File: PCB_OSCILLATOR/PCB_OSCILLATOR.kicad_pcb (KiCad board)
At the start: 2 copper layers, 67 parts, among them J1 Jumper, J10 Jumper, J11 Jumper, J2 Jumper, J3 Jumper, J4 Jumper, J5 Jumper, J6 Jumper, J7 Jumper, J8 Jumper, J9 Jumper, P1 POWER SUPPLY, P2 SPI_AD5270_1, P3 SPI_AD5270_2, P4 SPI_AD9833_1, P5 SPI_AD9833_2, U1 AD5270, U2 AD8421, U3 AD9833, U4 AD5270, U5 AD8421, U6 AD9833, U7 ADG819

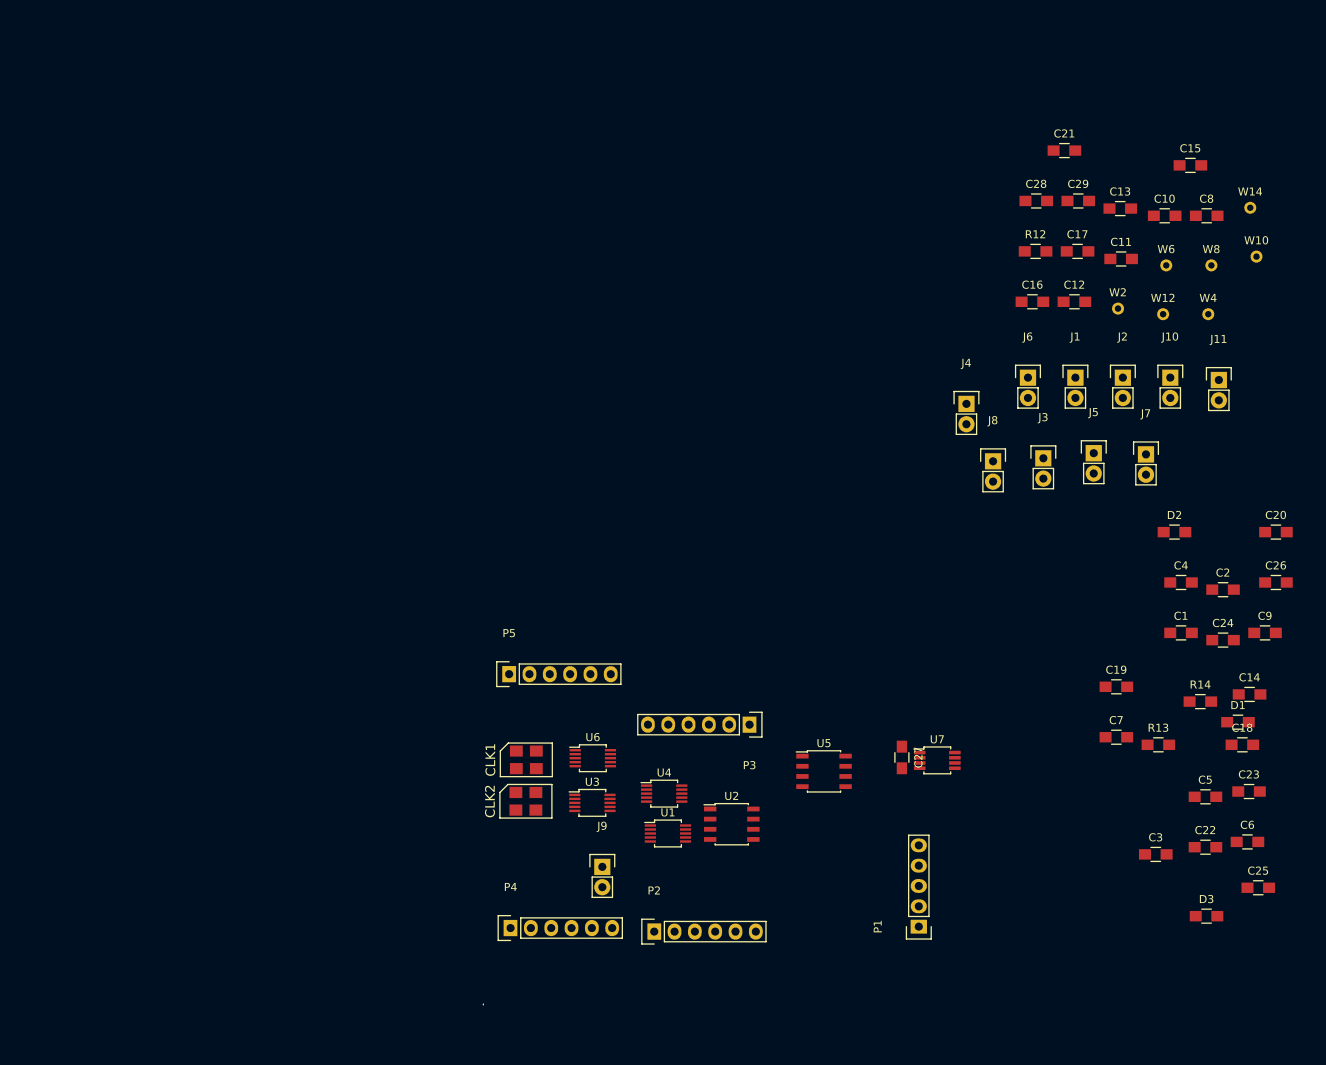
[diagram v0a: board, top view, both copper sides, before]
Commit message: Algunos cambios Adicionales
//
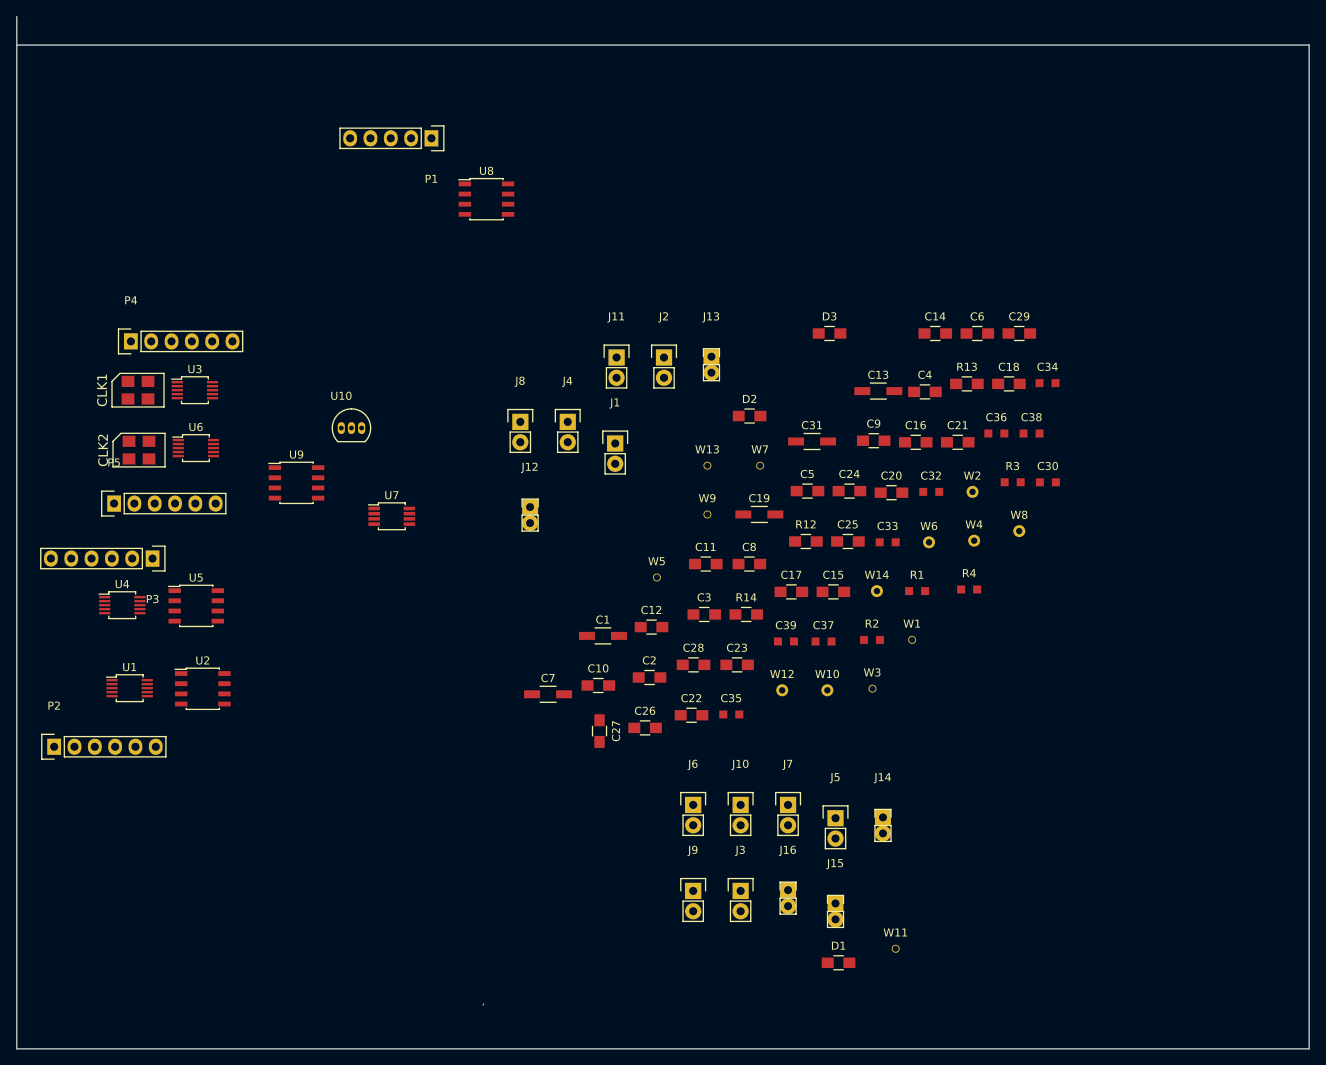
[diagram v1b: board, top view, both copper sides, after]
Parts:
- added C30: 1uF, Capacitors_SMD:C_0805_HandSoldering, F.Cu at (249.5, 97.4)
- added C31: 0.47uF, Capacitors_SMD:C_1206_HandSoldering, F.Cu at (220.0, 92.3)
- added C32: 0.1uF, Resistors_SMD:R_0805_HandSoldering, F.Cu at (234.9, 98.6)
- added C33: 0.1uF, Resistors_SMD:R_0805_HandSoldering, F.Cu at (229.5, 104.9)
- added C34: 10uF, Resistors_SMD:R_0805_HandSoldering, F.Cu at (249.5, 85.0)
- added C35: 0.1uF, Resistors_SMD:R_0805_HandSoldering, F.Cu at (209.9, 126.4)
- added C36: 10uF, Resistors_SMD:R_0805_HandSoldering, F.Cu at (243.1, 91.3)
- added C37: 0.1uF, Resistors_SMD:R_0805_HandSoldering, F.Cu at (221.5, 117.3)
- added C38: 10uF, Resistors_SMD:R_0805_HandSoldering, F.Cu at (247.5, 91.3)
- added C39: 0.1uF, Resistors_SMD:R_0805_HandSoldering, F.Cu at (216.8, 117.3)
- added J12: Jumper, Pin_Headers:Pin_Header_Straight_1x02, F.Cu at (184.8, 100.5)
- added J13: Jumper, Pin_Headers:Pin_Header_Straight_1x02, F.Cu at (207.4, 81.7)
- added J14: Jumper, Pin_Headers:Pin_Header_Straight_1x02, F.Cu at (228.9, 139.3)
- added J15: Jumper, Pin_Headers:Pin_Header_Straight_1x02, F.Cu at (223.0, 150.0)
- added J16: Jumper, Pin_Headers:Pin_Header_Straight_1x02, F.Cu at (217.0, 148.3)
- added R1: 1K, Resistors_SMD:R_0805_HandSoldering, F.Cu at (233.1, 111.0)
- added R2: 100K, Resistors_SMD:R_0805_HandSoldering, F.Cu at (227.5, 117.1)
- added R3: 1K, Resistors_SMD:R_0805_HandSoldering, F.Cu at (245.1, 97.4)
- added R4: 10K, Resistors_SMD:R_0805_HandSoldering, F.Cu at (239.7, 110.8)
- added U10: ADR291, TO_SOT_Packages_THT:TO-92_Inline_Narrow_Oval, F.Cu at (161.2, 90.6)
- added U8: ADP3303, Housings_SOIC:SOIC-8_3.9x4.9mm_Pitch1.27mm, F.Cu at (179.3, 62.0)
- added U9: AD8651, Housings_SOIC:SOIC-8_3.9x4.9mm_Pitch1.27mm, F.Cu at (155.6, 97.4)
- added W1: TEST_8, Measurement_Points:Measurement_Point_Round-TH_Small, F.Cu at (232.5, 117.1)
- added W11: TEST_13, Measurement_Points:Measurement_Point_Round-TH_Small, F.Cu at (230.5, 155.7)
- added W13: TEST_14, Measurement_Points:Measurement_Point_Round-TH_Small, F.Cu at (206.9, 95.3)
- added W3: TEST_9, Measurement_Points:Measurement_Point_Round-TH_Small, F.Cu at (227.6, 123.2)
- added W5: TEST_10, Measurement_Points:Measurement_Point_Round-TH_Small, F.Cu at (200.6, 109.3)
- added W7: TEST_11, Measurement_Points:Measurement_Point_Round-TH_Small, F.Cu at (213.5, 95.3)
- added W9: TEST_12, Measurement_Points:Measurement_Point_Round-TH_Small, F.Cu at (206.9, 101.4)
- C1, C13, C19, C7: footprint Resistors_SMD:R_0805_HandSoldering -> Capacitors_SMD:C_1206_HandSoldering
- moved P1 115.9 mm to (172.4, 54.4), turned to 180 degrees
- moved C10 92.0 mm to (193.3, 122.8)
- moved P4 87.3 mm to (134.9, 79.8)
- moved D3 86.7 mm to (222.2, 78.8)
- moved U5 81.2 mm to (143.0, 112.8)
- moved C26 80.9 mm to (199.2, 128.1)
- moved P2 78.5 mm to (125.3, 130.4)
- moved P3 77.5 mm to (137.6, 106.9)
- moved W10 76.3 mm to (221.9, 123.4)
- moved J10 75.7 mm to (211.1, 137.7)
- moved J11 75.3 mm to (195.6, 81.8)
- moved U7 74.7 mm to (167.5, 101.6)
- moved C2 72.5 mm to (199.7, 121.8)
- moved C1 72.3 mm to (193.9, 116.6)
- moved C28 72.1 mm to (205.2, 120.2)
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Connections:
- net /+18V renamed /+12V
- net /-18V renamed /-12V
- net /WAVE_AD8421_1 renamed /BASE_WAVE
- net /WAVE_AD8421_2 renamed /FINAL_WAVE
- C28 pad 1: /VDD -> /+5V
- C29 pad 1: /VDD -> /+5V
- CLK1 pad 1: /VDD -> Net-(CLK1-Pad1)
- CLK2 pad 1: /VDD -> Net-(CLK2-Pad1)
- D2 pad 2: /VDD -> /+5V
- P1 pad 1: /VDD -> /+5V
- U2 pad 6: /GND -> Net-(J12-Pad1)
- U5 pad 6: /GND -> Net-(J13-Pad1)
- U7 pad 6: /WAVE_DDS_2 -> /MODULATING_WAVE
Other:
- board outline added: 161.6 x 129 mm
